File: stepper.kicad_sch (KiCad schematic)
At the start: 32 parts, among them U6 TMC2209-LA, U7 TMC2209-LA

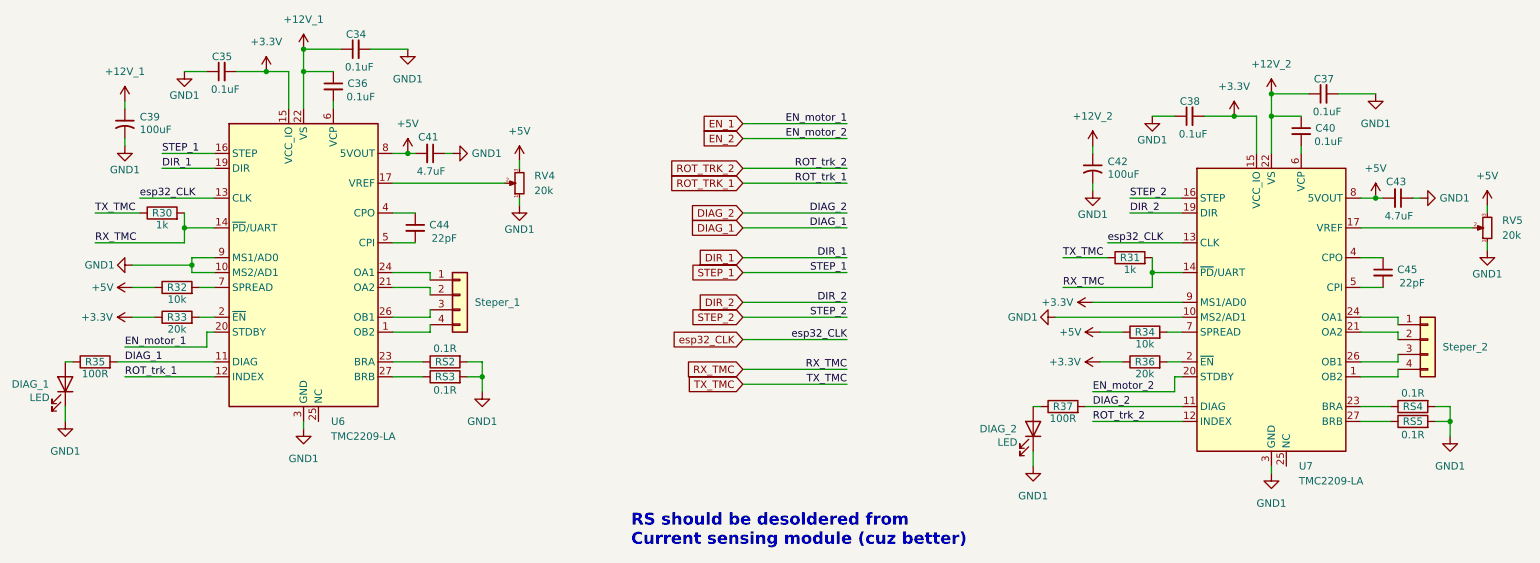
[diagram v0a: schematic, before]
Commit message: post production fixes
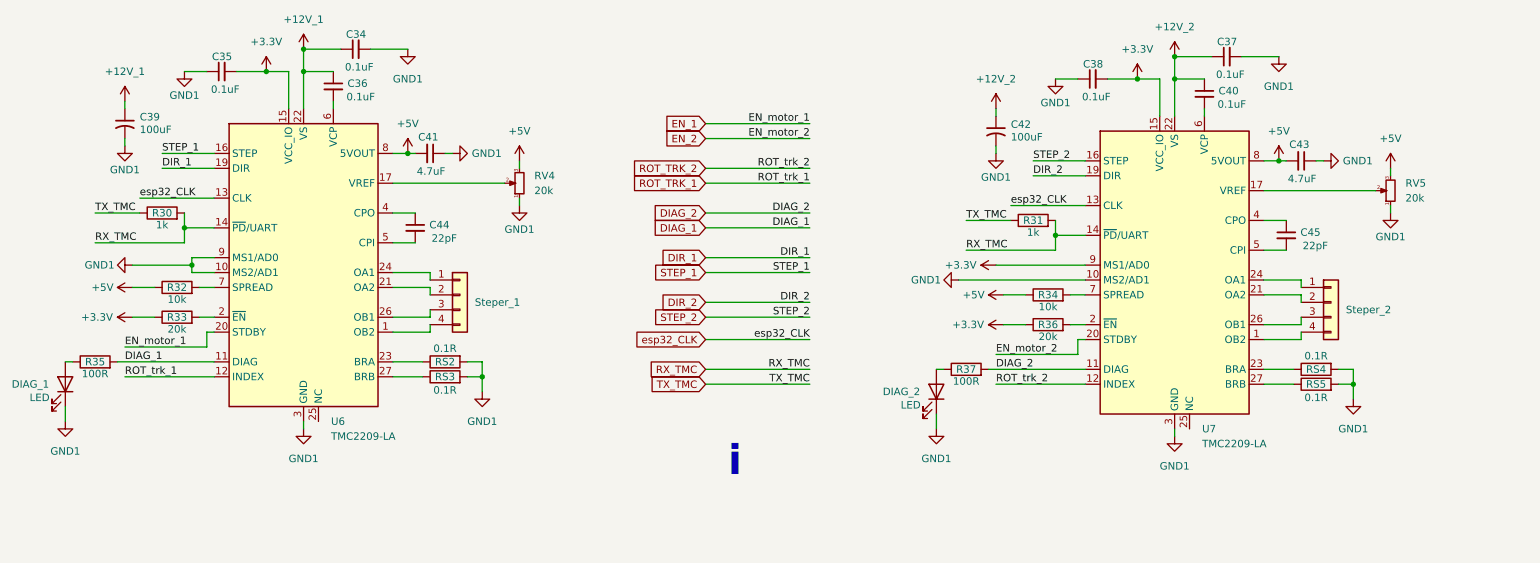
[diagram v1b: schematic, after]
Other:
- note added: "i"
- note removed: "RS should be desoldered from Current sensing module (cuz better)"
- moved on the sheet: C37, C38, C40, C42, C43, C45, DIAG_2, R31, R34, R36, R37, RS4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
